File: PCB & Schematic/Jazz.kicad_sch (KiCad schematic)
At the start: 29 parts, among them P1 MountingHole_Pad, U1 XIAO-nRF52840-DIP, U2 TLV75533PDBVR, U3 BQ24040DSQT, U4 MAX98357AETE+T

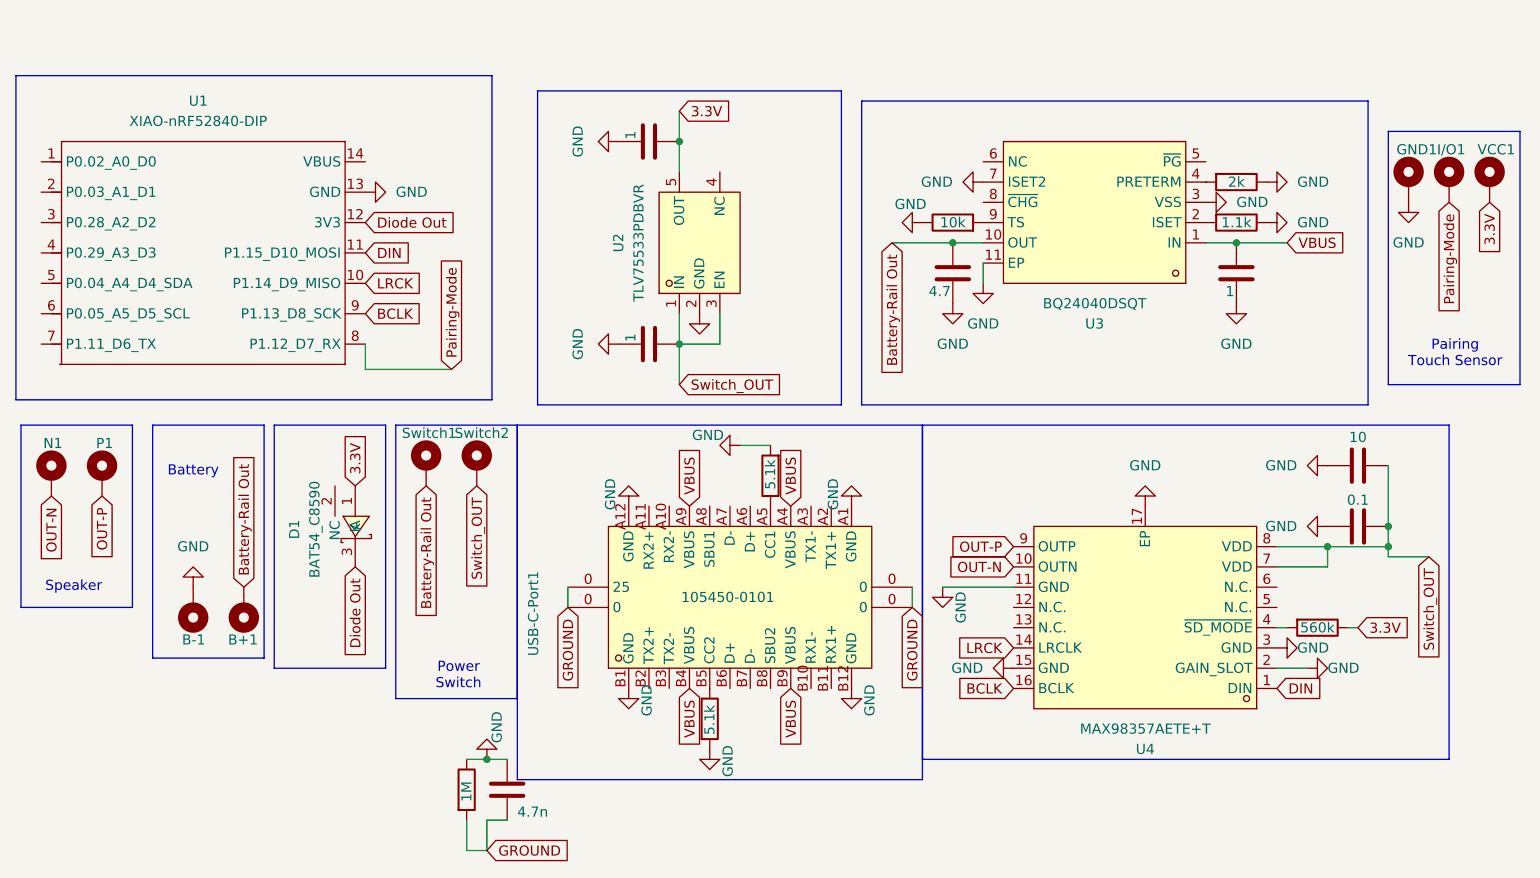
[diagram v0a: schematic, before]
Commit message: Possibly Done
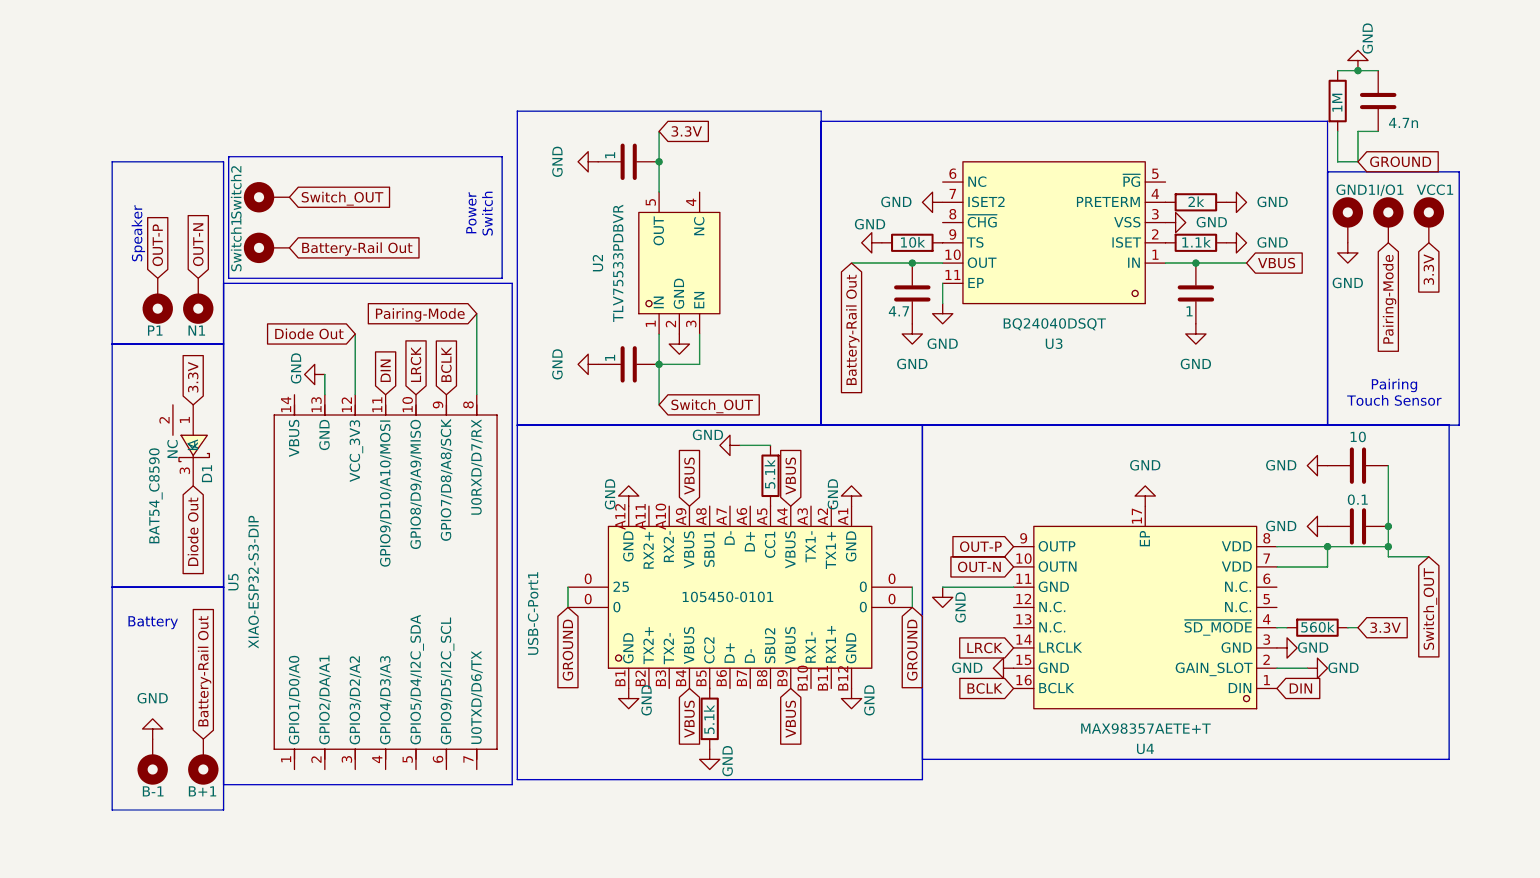
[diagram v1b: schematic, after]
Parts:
- removed U1: XIAO-nRF52840-DIP, Seeed Studio XIAO Series Library:XIAO-Generic-Thruhole-14P-2.54-21X17.8MM, symbol Snapeda:XIAO-nRF52840-DIP
- added U5: XIAO-ESP32-S3-DIP, Seeed Studio XIAO Series Library:XIAO-Generic-Thruhole-14P-2.54-21X17.8MM, symbol Seeed_Studio_XIAO_Series:XIAO-ESP32-S3-DIP
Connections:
- net BCLK: now also U5.9 (GPIO7/D8/A8/SCK)
- net DIN: now also U5.11 (GPIO9/D10/A10/MOSI)
- net Diode Out: now also U5.12 (VCC_3V3)
- net GND: now also U5.13 (GND)
- net LRCK: now also U5.10 (GPIO8/D9/A9/MISO)
- net Pairing-Mode: now also U5.8 (U0RXD/D7/RX)
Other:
- moved on the sheet: B+1, B-1, D1, GND1, I/O1, N1, P1, Switch1, Switch2, U2, U3, VCC1
